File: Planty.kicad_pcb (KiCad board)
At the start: 2 copper layers, 40.6 x 27.9 mm, 41 parts, among them J1 USB_C_Receptacle_USB2.0, Q1 WPM2031, U1 ESP32-C3, U2 MCP73831-2-OT, U3 MIC5504-3.3YM5, Y1 Crystal_GND24

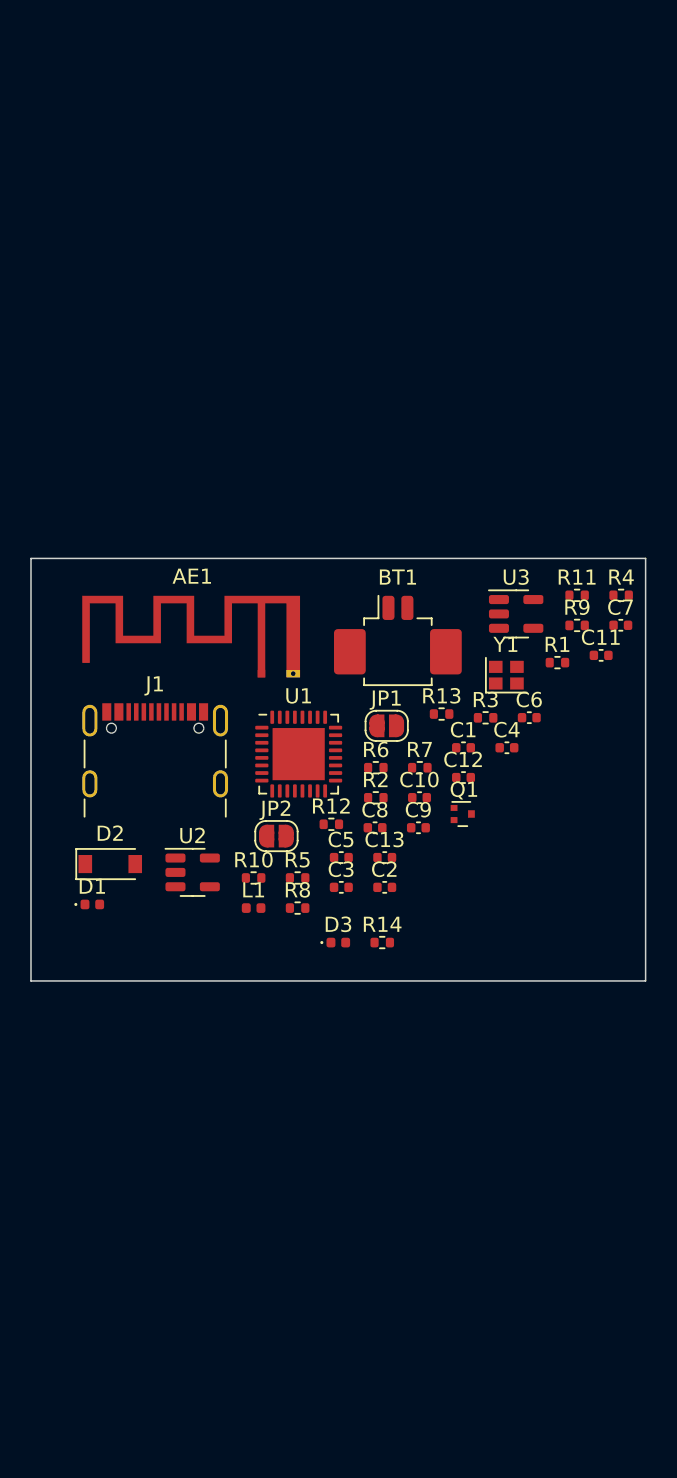
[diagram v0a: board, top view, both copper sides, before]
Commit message: finished v1.0.0
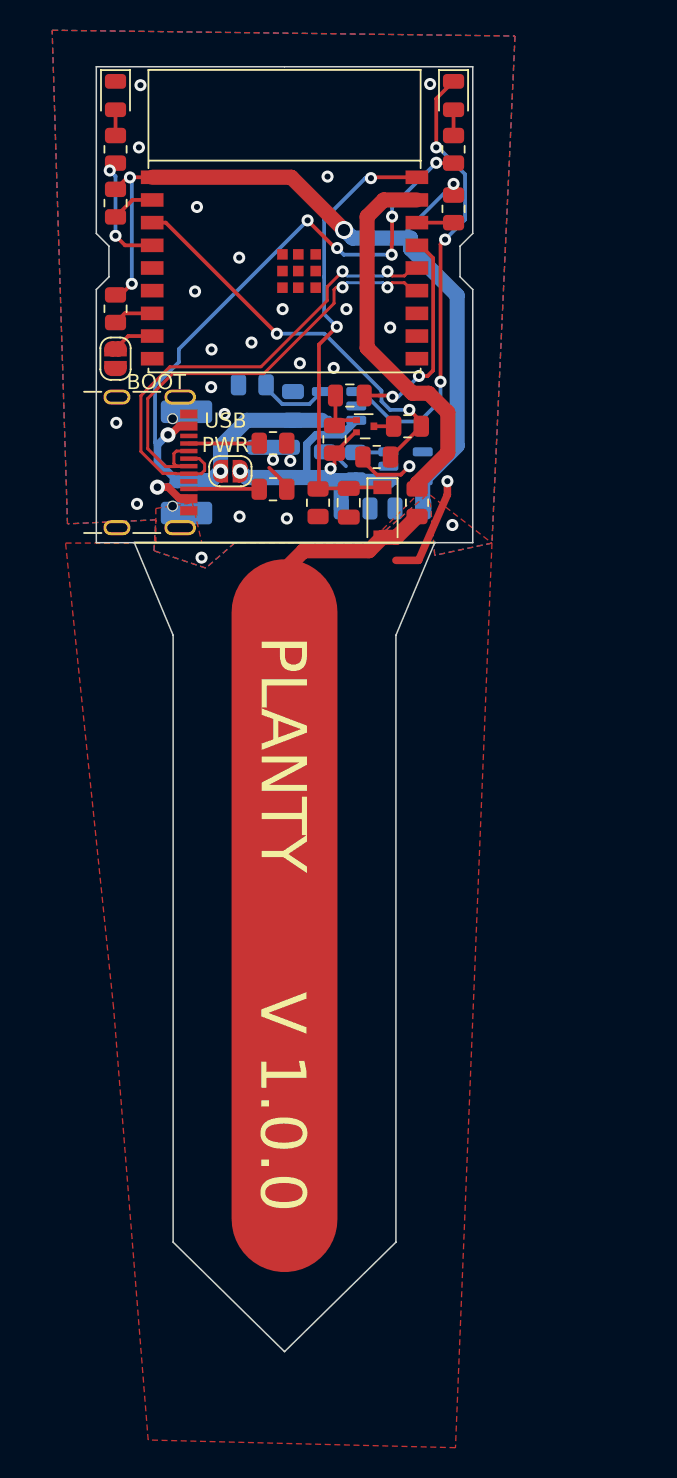
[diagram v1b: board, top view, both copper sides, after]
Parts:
- removed AE1: Antenna_Chip, RF_Antenna:Texas_SWRA117D_2.4GHz_Left
- removed C1, C3: 10p, Capacitor_SMD:C_0402_1005Metric
- removed C2, C4: 3p3, Capacitor_SMD:C_0402_1005Metric
- removed C5: 10u, Capacitor_SMD:C_0402_1005Metric
- removed C6, C7: 100n, Capacitor_SMD:C_0402_1005Metric
- removed L1: 2n2, Inductor_SMD:L_0402_1005Metric
- removed Y1: Crystal_GND24, Crystal:Crystal_SMD_2016-4Pin_2.0x1.6mm
- BT1: footprint Connector_Molex:Molex_PicoBlade_53261-0271_1x02-1MP_P1.25mm_Horizontal -> Connector_JST:JST_PH_S2B-PH-SM4-TB_1x02-1MP_P2.00mm_Horizontal; moved to B.Cu
- C10, C12, C8, C9: footprint Capacitor_SMD:C_0402_1005Metric -> Capacitor_SMD:C_0805_2012Metric; moved to B.Cu
- C11, C13: footprint Capacitor_SMD:C_0402_1005Metric -> Capacitor_SMD:C_0805_2012Metric
- D1, D3: footprint LED_SMD:LED_0402_1005Metric -> LED_SMD:LED_0805_2012Metric
- R1, R10, R11, R12, R13, R14, R2, R3, R5, R6, R7, R9: footprint Resistor_SMD:R_0402_1005Metric -> Resistor_SMD:R_0805_2012Metric
- R4: value 3k -> 10k; footprint Resistor_SMD:R_0402_1005Metric -> Resistor_SMD:R_0805_2012Metric; moved to B.Cu
- R8: footprint Resistor_SMD:R_0402_1005Metric -> Resistor_SMD:R_0805_2012Metric; moved to B.Cu
- U1: value ESP32-C3 -> ESP32-C3-WROOM-02; footprint Package_DFN_QFN:QFN-32-1EP_5x5mm_P0.5mm_EP3.45x3.45mm -> Espressif:ESP32-C3-WROOM-02
- U2, U3: moved to B.Cu
- moved D1 58.6 mm to (114.3, 22.7), turned to -90 degrees
- moved D3 57.9 mm to (91.9, 22.7), turned to -90 degrees
- moved R14 55.3 mm to (91.9, 26.3), turned to 90 degrees
- moved R5 49.3 mm to (114.3, 26.3), turned to 90 degrees
- moved R3 41.9 mm to (91.9, 29.8), turned to -90 degrees
- moved R7 37.0 mm to (114.3, 30.2), turned to -90 degrees
- moved R6 34.9 mm to (91.9, 36.8), turned to -90 degrees
- moved JP2 33.3 mm to (91.9, 40.1), turned to -90 degrees
- moved U2 32.3 mm to (106.7, 43.3), turned to 180 degrees
- moved U1 32.3 mm to (103.1, 34.0)
- moved R10 31.6 mm to (111.3, 44.6), turned to 180 degrees
- moved C13 30.6 mm to (107.4, 42.6), turned to 180 degrees
- moved R8 29.5 mm to (107.8, 47.2), turned to 90 degrees
- moved D2 29.4 mm to (109.6, 50.3), turned to -90 degrees
- moved C8 28.4 mm to (103.7, 43.3), turned to -90 degrees
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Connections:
- J1 pad S1: unconnected-(J1-PadS1) -> GND
- R14 pad 1: Net-(U1-Pad10) -> Net-(R14-Pad1)
- R6 pad 1: Net-(R6-Pad1) -> +3V3
- R6 pad 2: +3V3 -> Net-(R6-Pad2)
- R7 pad 1: Net-(R7-Pad1) -> +3V3
- R7 pad 2: +3V3 -> Net-(R7-Pad2)
- U1 pad 1: /Antenna -> +3V3
- U1 pad 10: Net-(U1-Pad10) -> unconnected-(U1-Pad10)
- U1 pad 11: +3V3 -> unconnected-(U1-Pad11)
- U1 pad 13: unconnected-(U1-Pad13) -> /D-
- U1 pad 14: Net-(R6-Pad1) -> /D+
- U1 pad 15: Net-(JP2-Pad1) -> /ADC_EN
- U1 pad 16: unconnected-(U1-Pad16) -> Net-(R7-Pad2)
- U1 pad 17: +3V3 -> /PULSE
- U1 pad 18: unconnected-(U1-Pad18) -> /OUT
- U1 pad 19: unconnected-(U1-Pad19) -> GND
- U1 pad 2: +3V3 -> Net-(R3-Pad2)
- U1 pad 3: +3V3 -> /ADC
- U1 pad 4: /OUT -> Net-(R14-Pad1)
- U1 pad 5: /PULSE -> unconnected-(U1-Pad5)
- U1 pad 6: Net-(R7-Pad1) -> unconnected-(U1-Pad6)
- U1 pad 7: Net-(R3-Pad2) -> Net-(R6-Pad2)
- U1 pad 8: /ADC_EN -> Net-(JP2-Pad1)
- U1 pad 9: /ADC -> GND
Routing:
- net +3V3: track 0.00 -> 55.8 mm, vias 0 -> 4
- net VBUS: track 0.00 -> 55.3 mm, vias 0 -> 8
- net Net-(D2-Pad2): track 0.00 -> 53.2 mm
- net /D+: track 0.00 -> 33.0 mm, vias 0 -> 2
- net /D-: track 0.00 -> 31.3 mm, vias 0 -> 2
- net /OUT: track 0.00 -> 30.3 mm, vias 0 -> 2
- net Net-(D1-Pad1): track 0.00 -> 30.1 mm, vias 0 -> 3
- net /ADC: track 0.00 -> 26.8 mm, vias 0 -> 2
- net /PULSE: track 0.00 -> 25.4 mm
- net +BATT: track 0.00 -> 21.8 mm, vias 0 -> 2
- net GND: track 0.00 -> 14.8 mm, vias 0 -> 26
- net /ADC_EN: track 0.00 -> 14.2 mm, vias 0 -> 2
- net Net-(R14-Pad1): track 0.00 -> 7.81 mm, vias 0 -> 2
- net Net-(R4-Pad2): track 0.00 -> 4.68 mm
- net Net-(J1-PadB5): track 0.00 -> 4.66 mm
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- added copper zone on B.Cu, net GND
- added copper zone on F.Cu, net GND
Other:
- board size 40.6 x 27.9 mm -> 24.9 x 85 mm
- board text added: "+"
- board text added: "BATTERY"
- board text added: "BOOT"
- board text added: "PLACE BATTERY HERE"
- board text added: "PLANTY"
- board text added: "Philipp Tebbe - 2023 github.com/phsete/planty"
- board text added: "USB PWR"
- board text added: "V 1.0.0"
